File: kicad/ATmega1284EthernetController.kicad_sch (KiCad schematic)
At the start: 43 parts, among them J1 AVR-ISP-6, J2 PA0-7, J3 PC0-7, J4 PB0-3/PD3-7, J5 DC 9-12V, J6 SIO, J7 RJ45_Amphenol_RJMG1BD3B8K1ANR, SW1 RESET, U1 ATmega1284P-A, U2 74HCT32, U3 ENC28J60x-SP, U4 LM7805_TO220, Y1 20MHz, Y2 25MHz

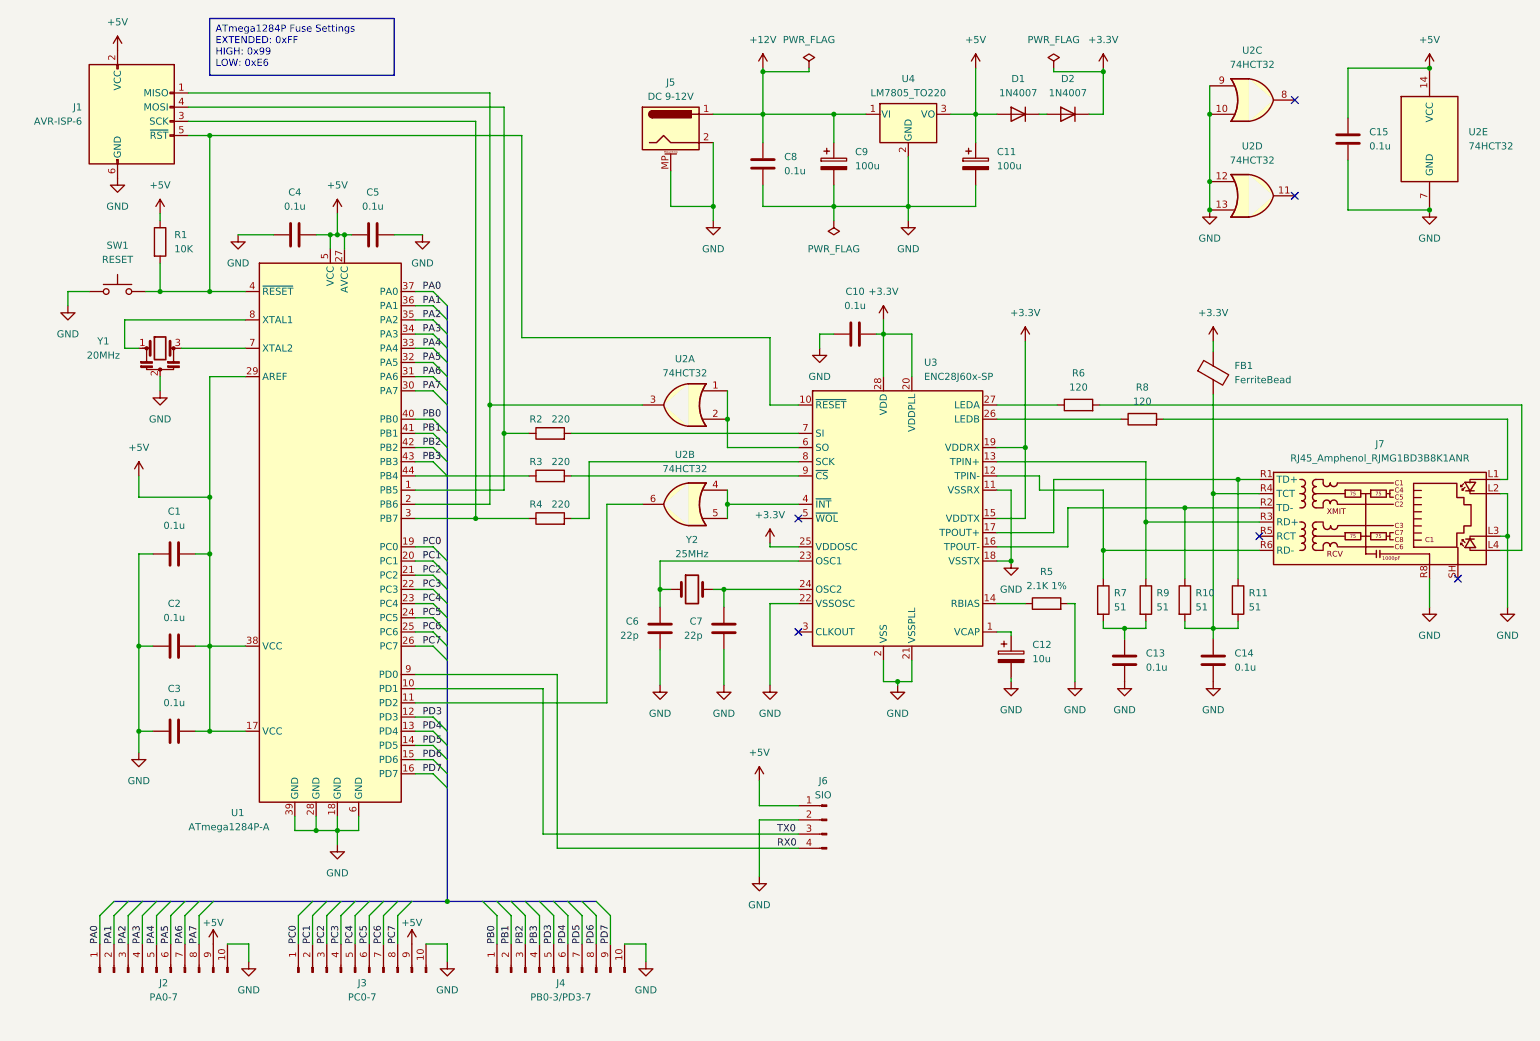
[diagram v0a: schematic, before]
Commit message: PCB base
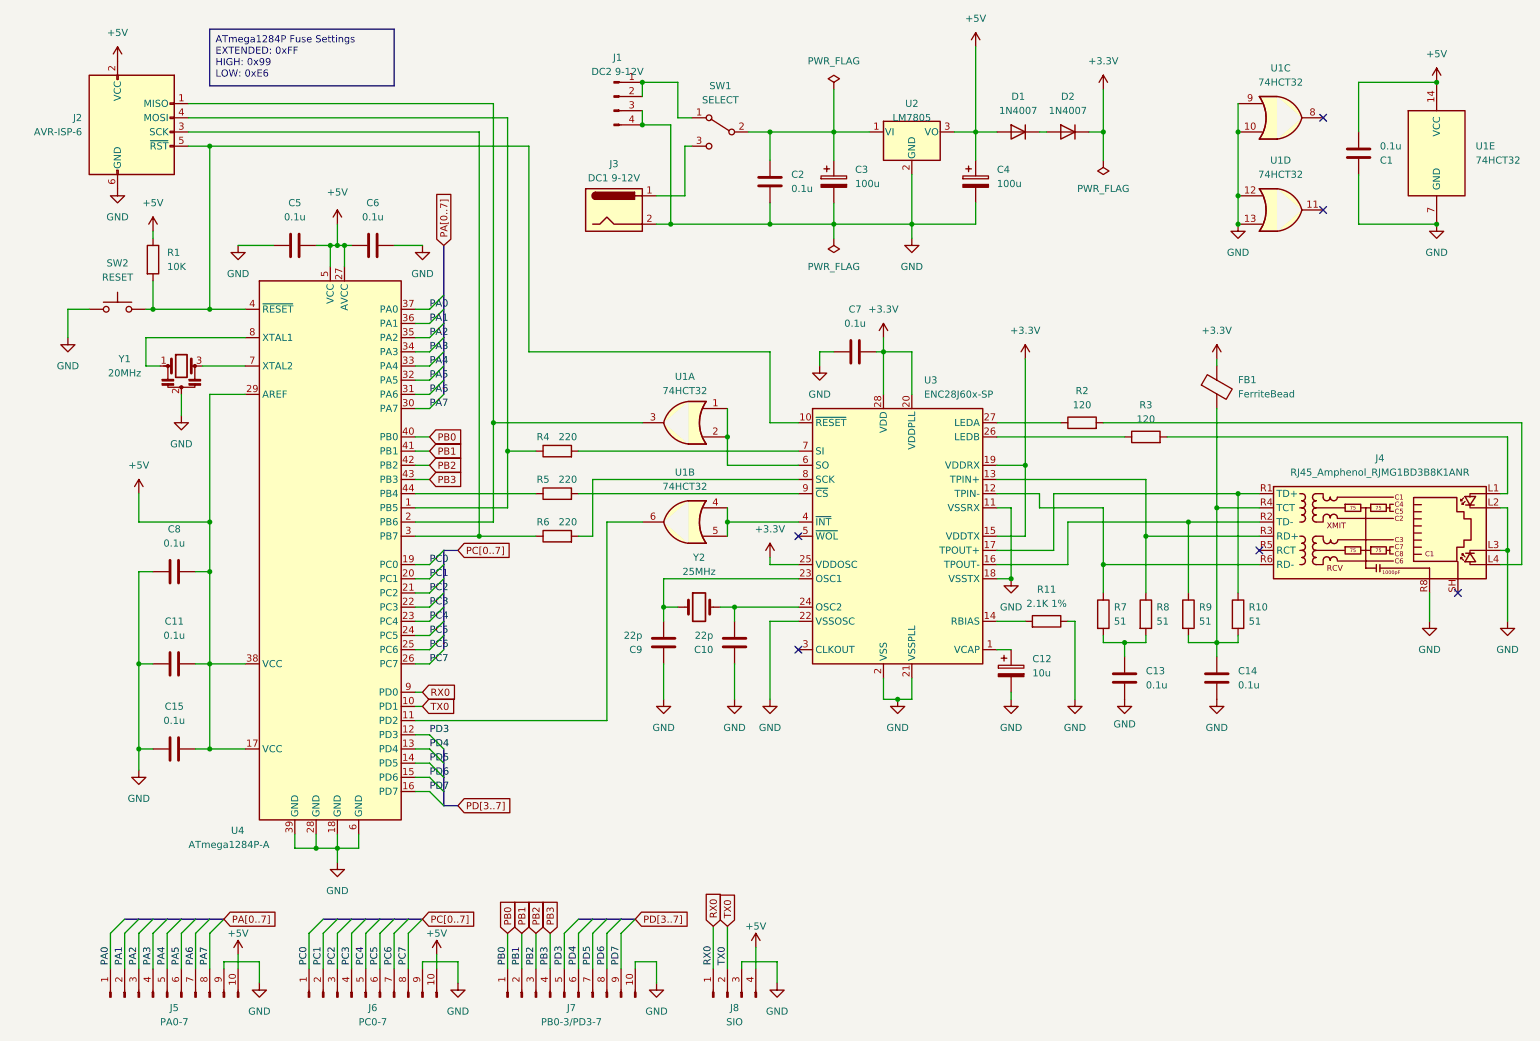
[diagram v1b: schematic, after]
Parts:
- removed J5: DC 9-12V, Connector_BarrelJack:BarrelJack_Horizontal, symbol Connector:Barrel_Jack_MountingPin
- removed J6: SIO, Connector_PinHeader_2.54mm:PinHeader_1x04_P2.54mm_Vertical, symbol Connector:Conn_01x04_Pin
- removed U4: LM7805_TO220, Package_TO_SOT_THT:TO-220-3_Vertical, symbol Regulator_Linear:LM7805_TO220
- added J1: DC2 9-12V, Connector_PinHeader_2.00mm:PinHeader_1x04_P2.00mm_Vertical, symbol Connector:Conn_01x04_Pin
- added J3: DC1 9-12V, Connector_BarrelJack:BarrelJack_Horizontal, symbol Connector:Barrel_Jack
- added J8: SIO, Connector_PinHeader_2.54mm:PinHeader_1x04_P2.54mm_Vertical, symbol Connector:Conn_01x04_Pin
- added SW1: SELECT, Button_Switch_THT:SW_Slide_1P2T_CK_OS102011MS2Q, symbol Switch:SW_SPDT
- added U2: LM7805, Package_TO_SOT_THT:TO-220-3_Vertical, symbol Regulator_Linear:LM7805_TO220
- renumbered C15 to C1, C7 to C10, C2 to C11, C3 to C15, C8 to C2, C9 to C3, C11 to C4, C4 to C5, C5 to C6, C10 to C7, C1 to C8, C6 to C9, J1 to J2, J7 to J4, J2 to J5, J3 to J6, J4 to J7, R11 to R10, R5 to R11, R6 to R2, R8 to R3, R2 to R4, R3 to R5, R4 to R6, R9 to R8, R10 to R9, SW1 to SW2, U2 to U1, U1 to U4
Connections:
- net +5V: now also C1.2, C11.2, J5.10 (Pin_10), J6.10 (Pin_10), J8.4 (Pin_4), U2.3 (VO); no longer C1.1, C11.1, J5.9 (Pin_9), J6.9 (Pin_9)
- net GND: now also C1.1, C10.1, C11.1, C9.1, J5.9 (Pin_9), J6.9 (Pin_9), R11.1, J1.3 (Pin_3), J1.4 (Pin_4), J3.2, J8.3 (Pin_3), U2.2 (GND); no longer C1.2, C10.2, C11.2, C9.2, J5.10 (Pin_10), J6.10 (Pin_10), R11.2
- net RX0: now also J8.1 (Pin_1)
- net TX0: now also J8.2 (Pin_2)
- net at U3.14 (RBIAS): now also R11.2; no longer R11.1
- net at U3.23 (OSC1), Y2.1: now also C9.2; no longer C9.1
- net at U3.24 (OSC2), Y2.2: now also C10.2; no longer C10.1
- net +12V: no longer names the net of C2.1, C3.1
- net +12V: now also SW1.2 (B), U2.1 (VI)
- new net: J1.1 (Pin_1), J1.2 (Pin_2), SW1.1 (A)
- new net: J3.1, SW1.3 (C)
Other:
- moved on the sheet: C1, C10, C11, C12, C13, C14, C15, C2, C3, C4, C5, C6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
